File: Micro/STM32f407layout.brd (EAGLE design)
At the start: 36 x 76 mm, 40 parts, among them Q1 ASF, U1 LM1085IS-3.3

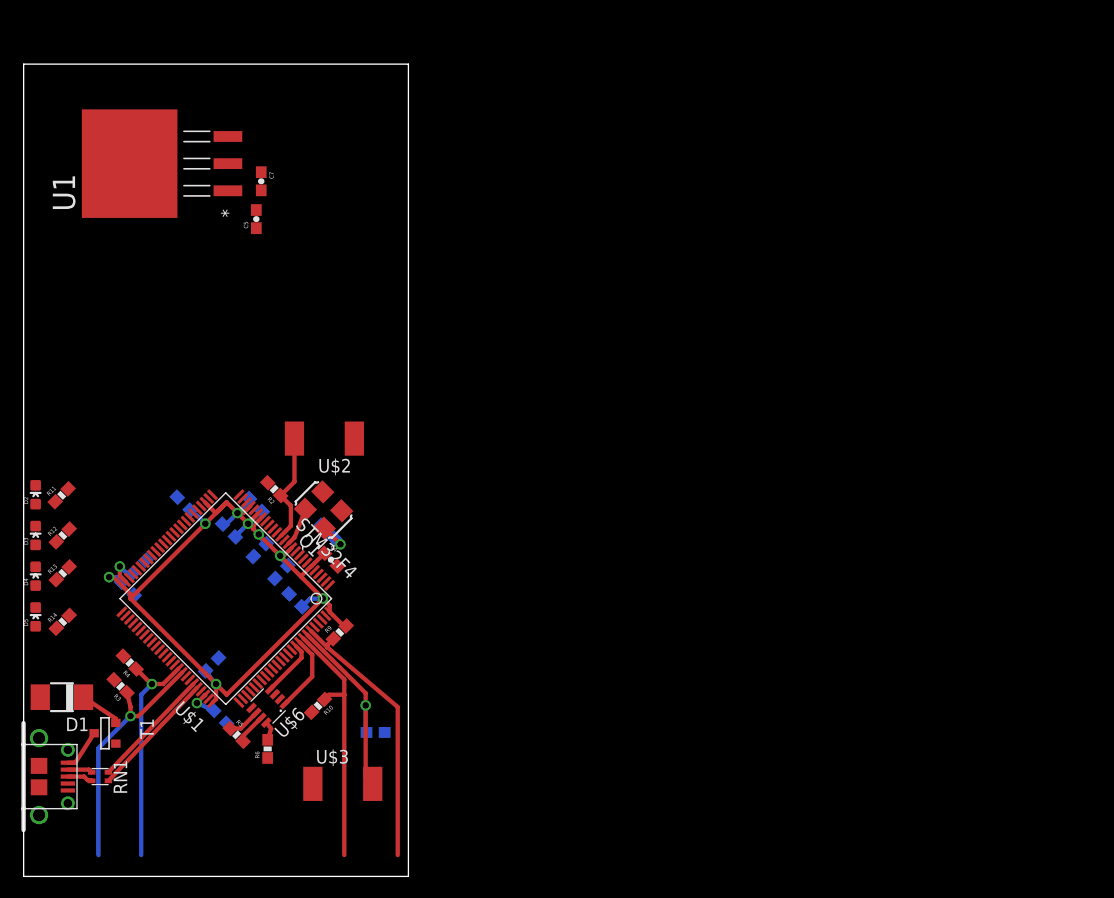
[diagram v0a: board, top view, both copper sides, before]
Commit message: Made changes to the micro board
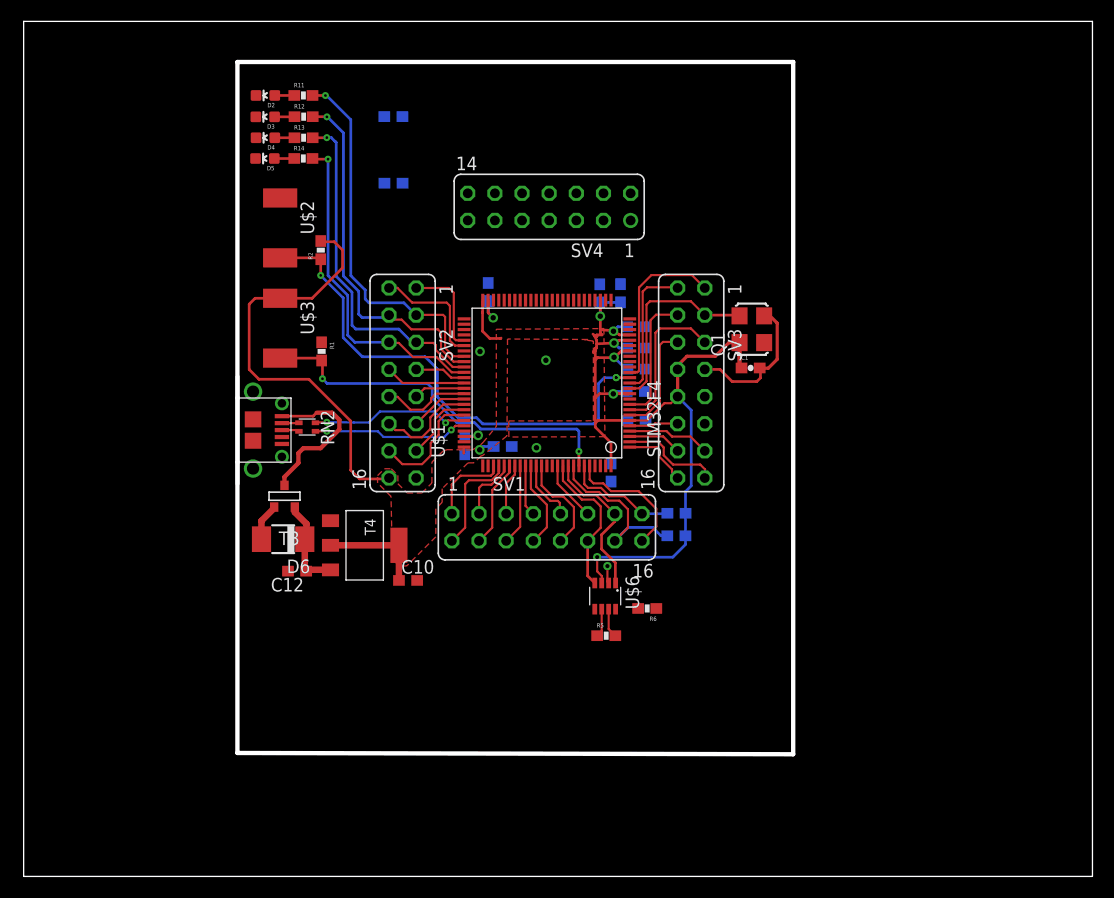
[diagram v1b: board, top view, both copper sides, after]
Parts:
- removed C5, C7: 0.22uF, SparkFun-Passives:0603-CAP
- removed D1: (no value), DiscreteComponents:DO-214AC
- removed RN1: (no value), DiscreteComponents:EXBV4V
- removed T1: (no value), DiscreteComponents:SOT-23
- removed U$4: MICROUSB, Other:MICRO_B
- removed U1: LM1085IS-3.3, PowerComponents:TO254P1435X457-3N
- added C10, C12: 0.22uF, rcl:C0603
- added D6: (no value), DiscreteComponents:DO-214AC
- added RN2: (no value), DiscreteComponents:EXBV4V
- added SV1, SV2, SV3: (no value), con-lsta:FE08-2
- added SV4: (no value), con-lsta:FE07-2
- added T3: FDN340P, DiscreteComponents:SOT-23
- added T4: AP1117_LIN_REG, PowerComponents:SOT223
- added U$5: MICROUSB, Other:MICRO_B
- moved C1 57.5 mm to (68.0, 47.6), flipped to the top, turned to 0 degrees
- moved R4 56.7 mm to (34.6, 71.1), flipped to the bottom, turned to 0 degrees
- moved C8 53.7 mm to (55.8, 54.6), turned to 90 degrees
- moved R3 53.5 mm to (34.6, 64.9), flipped to the bottom, turned to 0 degrees
- moved R14 48.8 mm to (26.2, 67.2), turned to 0 degrees
- moved D5 48.0 mm to (22.6, 67.2), turned to 90 degrees
- moved R13 46.6 mm to (26.2, 69.1), turned to 0 degrees
- moved D4 46.3 mm to (22.6, 69.1), turned to 90 degrees
- moved R12 45.2 mm to (26.2, 71.1), turned to 0 degrees
- moved D3 44.7 mm to (22.6, 71.1), turned to 90 degrees
- moved C11 44.2 mm to (57.3, 47.5), turned to 180 degrees
- moved R11 43.7 mm to (26.2, 73.1), turned to 0 degrees
- moved Q1 43.5 mm to (68.1, 51.2), turned to 90 degrees
- moved D2 43.1 mm to (22.6, 73.1), turned to 90 degrees
- moved U$3 43.0 mm to (24.0, 51.3), turned to 270 degrees
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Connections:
- removed net ETC_MDC: U$1.P16
- removed net ETH_CRS_DV: U$1.P32
- removed net ETH_MDIO: U$1.P25
- removed net ETH_REF_CLK: U$1.P24
- removed net ETH_RXD0: U$1.P33
- removed net ETH_RXD1: U$1.P34
- removed net ETH_TXD0: U$1.P51
- removed net ETH_TXD1: U$1.P52
- removed net ETH_TX_EN: U$1.P48
- removed net N$10: T1.1, U$4.P1
- removed net N$16: R13.2, U$1.P60
- removed net N$19: R11.2, U$1.P58
- removed net N$22: C17.2, C18.2, U$1.P20
- removed net N$5: D1.C, T1.2
- removed net N$6: RN1.2, U$4.P3
- removed net N$7: RN1.1, U$4.P2
- removed net N$8: R12.2, U$1.P59
- removed net N$9: R14.2, U$1.P61
- removed net VCC: U$6.3
- new net CRS_DV: SV4.7, U$1.P32
- new net MDC: SV4.5, U$1.P16
- new net MDIO: SV4.6, U$1.P25
- new net N$12: RN2.1, U$5.P2
- new net N$24: RN2.2, U$5.P3
- new net N$57: T3.1, U$5.P1
- new net N$58: C12.1, D6.C, T3.2, T4.VIN
- new net PA10: SV2.14, U$1.P69
- new net PA13: U$1.P72
- new net PA14: U$1.P76
- new net PA15: U$1.P77
- new net PA5: U$1.P31
- new net PA9: SV2.13, U$1.P68
- new net PB0: U$1.P35
- new net PB1: U$1.P36
- new net PB10: U$1.P47
- new net PB14: U$1.P53
- new net PB15: U$1.P54
- new net PB2: U$1.P37
- new net PB3: U$1.P89
- new net PB4: SV1.11, U$1.P90
- new net PB9: SV1.16, U$1.P96
- new net PC0: SV3.1, U$1.P15
- new net PC10: SV1.1, U$1.P78
- new net PC11: SV1.2, U$1.P79
- new net PC12: SV1.3, U$1.P80
- new net PC13: SV3.6, U$1.P7
- new net PC14: SV3.5, U$1.P8
- new net PC15: SV3.4, U$1.P9
- new net PC2: U$1.P17
- new net PC3: U$1.P18
- new net PC6: SV2.8, U$1.P63
- new net PC7: SV2.9, U$1.P64
- new net PC8: SV2.10, U$1.P65
- new net PD0: SV1.4, U$1.P81
- new net PD1: SV1.5, U$1.P82
- new net PD10: U$1.P57
- new net PD11: R11.2, SV2.3, U$1.P58
- new net PD12: R12.2, SV2.4, U$1.P59
- new net PD13: R13.2, SV2.5, U$1.P60
- new net PD14: R14.2, SV2.6, U$1.P61
- new net PD15: SV2.7, U$1.P62
- new net PD2: SV1.6, U$1.P83
- new net PD3: SV1.7, U$1.P84
- new net PD4: SV1.8, U$1.P85
- new net PD5: SV1.9, U$1.P86
- new net PD6: SV1.10, U$1.P87
- new net PD7: U$1.P88
- new net PD8: SV2.1, U$1.P55
- new net PD9: SV2.2, U$1.P56
- new net PE0: U$1.P97
- new net PE1: U$1.P98
- new net PE10: U$1.P41
- new net PE11: U$1.P42
- new net PE12: U$1.P43
- new net PE13: U$1.P44
- new net PE14: U$1.P45
- new net PE15: U$1.P46
- new net PE2: SV3.16, U$1.P1
- new net PE3: SV3.15, U$1.P2
- new net PE4: SV3.14, U$1.P3
- new net PE5: SV3.13, U$1.P4
- new net PE6: SV3.12, U$1.P5
- new net PE7: U$1.P38
- new net PE8: U$1.P39
- new net PE9: U$1.P40
- new net PH1: SV3.2, U$1.P13
- new net REFCLK: SV4.8, U$1.P24
- new net RXD0: SV4.10, U$1.P33
- new net RXD1: SV4.9, U$1.P34
- new net TXD0: SV4.11, U$1.P51
- new net TXD1: SV4.14, U$1.P52
- new net TXEN: SV4.12, U$1.P48
- net +3V3: now also C10.1, SV2.16, SV3.10, SV3.8, SV4.1, SV4.2, T4.TAB, T4.VOUT, U$6.3; no longer C7.1, U1.2, U1.4
- net +5V: now also D6.A, T3.3; no longer C5.1, D1.A, T1.3, U1.3
- net CAN_RX: now also SV1.12
- net CAN_TX: now also SV1.13
- net GND: now also C10.2, C12.2, C17.2, C18.2, SV2.15, SV3.11, SV3.7, SV3.9, SV4.3, SV4.4, T4.GND, U$1.P20, U$5.GND1, U$5.GND2, U$5.GND3, U$5.GND4, U$5.GND7, U$5.GND8, U$5.P4, U$5.P5; no longer C5.2, C7.2, U$4.GND1, U$4.GND2, U$4.GND3, U$4.GND4, U$4.GND7, U$4.GND8, U$4.P4, U$4.P5, U1.1
- net I2C1_SCL: now also SV1.15
- net I2C1_SDA: now also SV1.14
- net I2C3_SCL: now also SV2.12
- net I2C3_SDA: now also SV2.11
- net OSC_IN: now also SV3.3
- net USB_D+: now also RN2.3; no longer RN1.3
- net USB_D-: now also RN2.4; no longer RN1.4
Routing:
- net +3V3: track 85.9 -> 145.8 mm, vias 8 -> 7
- net N$4: track 10.5 -> 47.6 mm, vias 0 -> 3
- net PD11: track 0.00 -> 35.0 mm, vias 0 -> 1
- net PD12: track 0.00 -> 33.9 mm, vias 0 -> 1
- net PD13: track 0.00 -> 32.5 mm, vias 0 -> 1
- net PD14: track 0.00 -> 31.0 mm, vias 0 -> 1
- net N$3: track 19.1 -> 35.6 mm, vias 1 -> 2
- net I2C3_SDA: track 21.6 -> 5.44 mm, vias 1 -> 0
- net PC0: track 0.00 -> 15.8 mm
- net GND: track 0.00 -> 15.3 mm, vias 0 -> 1
- net I2C1_SCL: track 25.7 -> 10.6 mm
- net N$57: track 0.00 -> 15.0 mm
- net OSC_IN: track 3.68 -> 18.4 mm
- net PC14: track 0.00 -> 14.4 mm
- net I2C3_SCL: track 23.0 -> 9.46 mm, vias 1 -> 0
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- added copper zone on layer 1, net +3V3
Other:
- board size 36 x 76 mm -> 100 x 80 mm
